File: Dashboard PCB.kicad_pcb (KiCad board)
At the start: 2 copper layers, 200 x 100 mm, 59 parts, among them J1 Controls_Leader_Export_02x06, J3 INDICATOR_SWITCH_OUT, J4 FAN_CTRL_01x02, J5 Horn_In_01x02, J6 Horn_Out_01x02

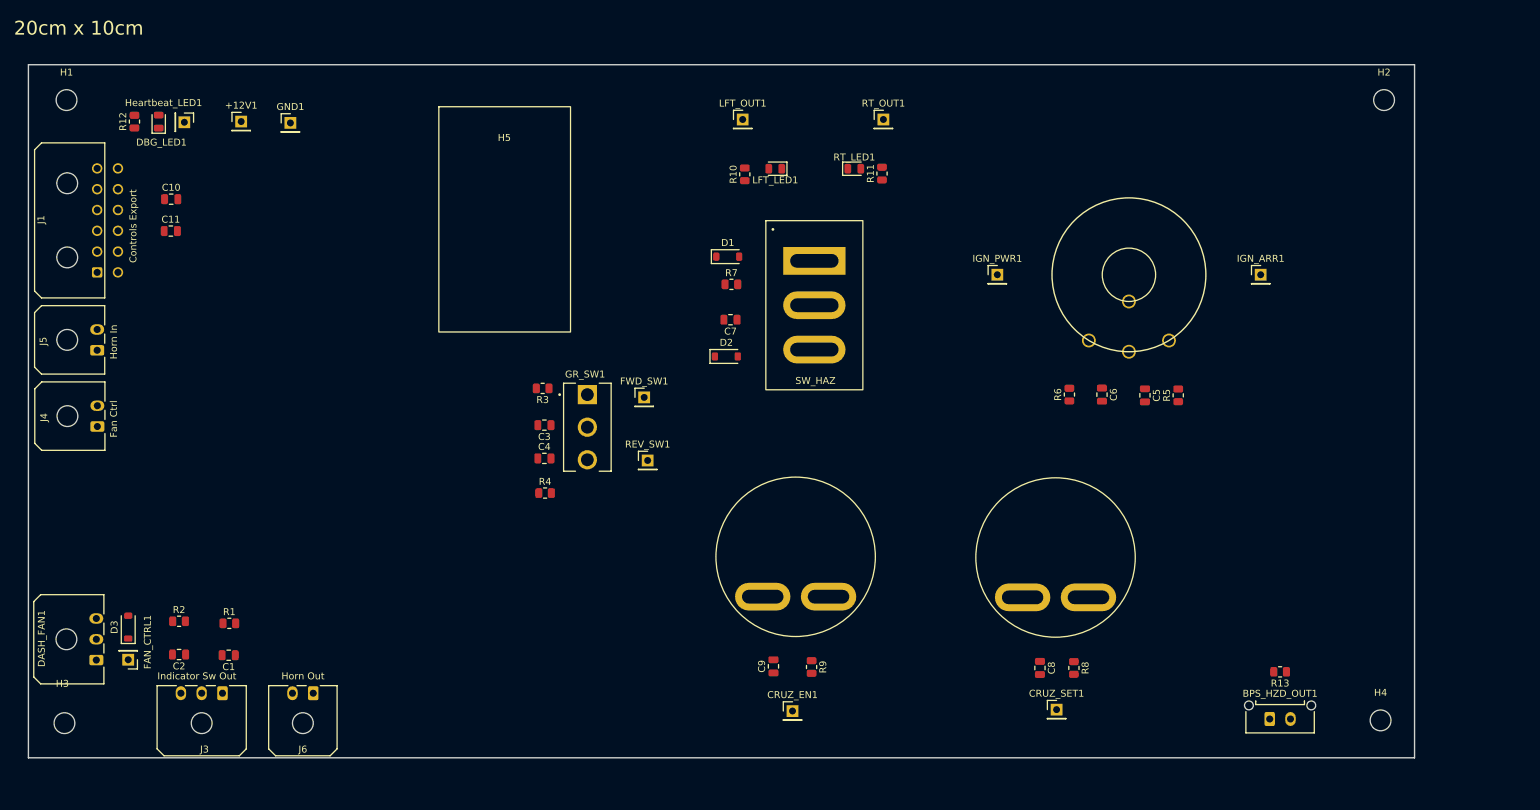
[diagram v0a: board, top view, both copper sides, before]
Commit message: Changed layout, added 3d models
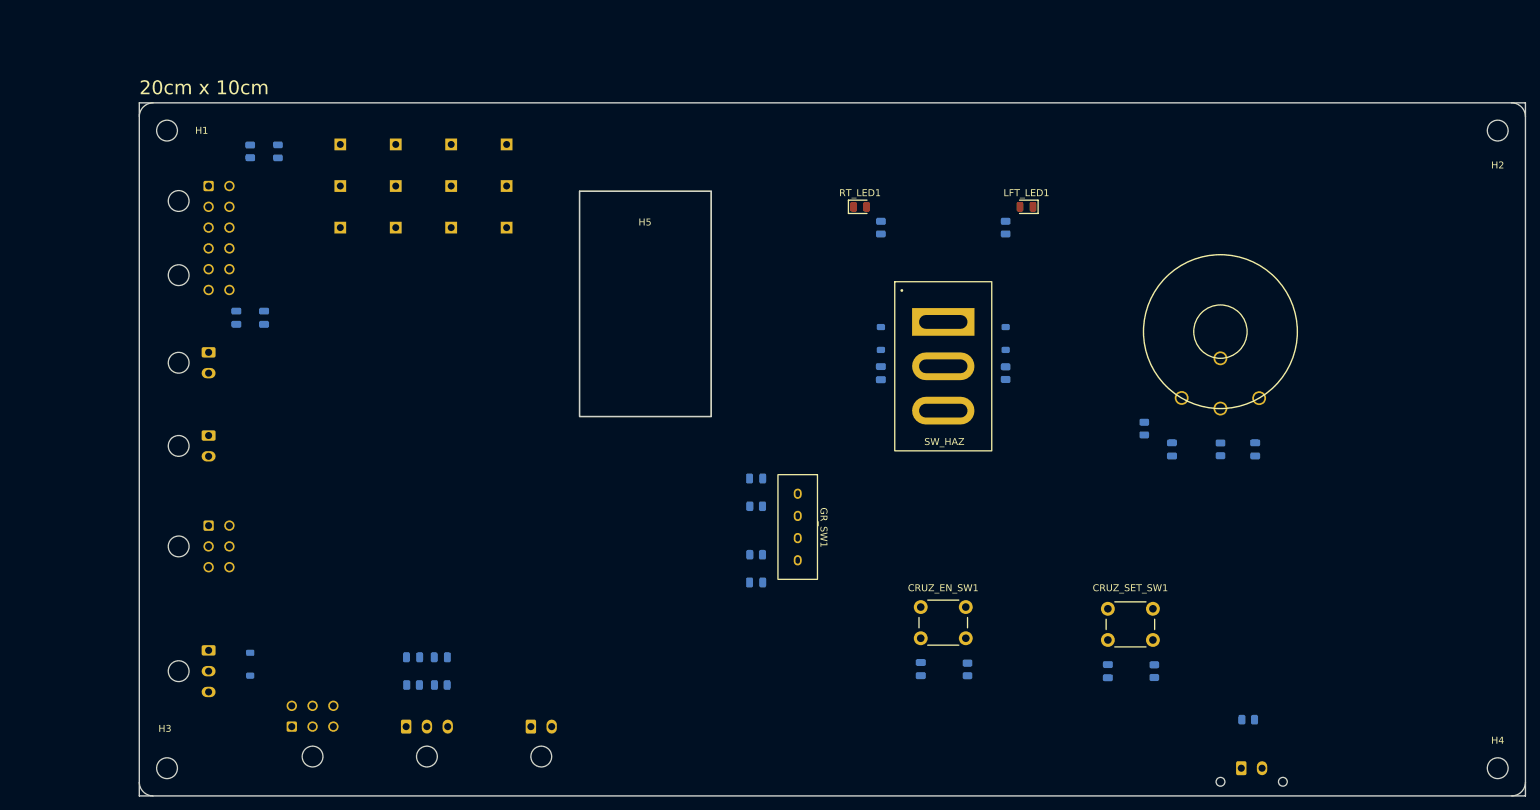
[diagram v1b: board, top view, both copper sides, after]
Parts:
- added J2: CAN, Connector_Molex:Molex_Micro-Fit_3.0_43045-0600_2x03_P3.00mm_Horizontal, B.Cu at (74.0, 104.0)
- added J7: CAN, Connector_Molex:Molex_Micro-Fit_3.0_43045-0600_2x03_P3.00mm_Horizontal, B.Cu at (86.0, 133.0)
- +12V1, BPS_HZD_OUT1, C1, C10, C11, C2, C3, C4, C5, C6, C7, C8, C9, CRUZ_EN1, CRUZ_SET1, D1, D2, D3, DASH_FAN1, DBG_LED1, FAN_CTRL1, FWD_SW1, GND1, Heartbeat_LED1, IGN_ARR1, IGN_PWR1, J1, J3, J4, J5, J6, LFT_OUT1, R1, R10, R11, R12, R13, R2, R3, R4, R5, R6, R7, R8, R9, REV_SW1, RT_OUT1: moved to B.Cu
- CRUZ_EN_SW1, CRUZ_SET_SW1: footprint switched:SW_Butt_) -> Button_Switch_THT:SW_PUSH_6mm
- GR_SW1: footprint switched:SW_100_SP3T-Vertical -> switched:3posSlideToggle
- moved IGN_ARR1 133.0 mm to (93.0, 61.0), turned to 180 degrees
- moved CRUZ_SET1 113.8 mm to (117.0, 49.0), turned to 180 degrees
- moved IGN_PWR1 95.7 mm to (93.0, 55.0), turned to 180 degrees
- moved CRUZ_EN1 86.3 mm to (117.0, 55.0), turned to 180 degrees
- moved FAN_CTRL1 73.3 mm to (101.0, 61.0), turned to -90 degrees
- moved RT_OUT1 56.6 mm to (117.0, 61.0), turned to 180 degrees
- moved LFT_OUT1 50.2 mm to (101.0, 49.0), turned to 180 degrees
- moved REV_SW1 48.7 mm to (109.0, 55.0), turned to 180 degrees
- moved R7 41.6 mm to (189.0, 82.0), turned to 90 degrees
- moved D2 40.4 mm to (189.0, 77.0), turned to -90 degrees
- moved R2 38.9 mm to (107.5, 127.0)
- moved R10 38.4 mm to (189.0, 61.0)
- moved C2 37.8 mm to (107.5, 123.0)
- moved FWD_SW1 37.1 mm to (109.0, 61.0), turned to 180 degrees
- moved LFT_LED1 36.7 mm to (192.0, 58.0)
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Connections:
- BPS_HZD_OUT1 pad 2: GND -> /BPS_HZD
- GR_SW1 pad 1: /FWD_SW -> +12V
- GR_SW1 pad 2: +12V -> /FWD_SW
- GR_SW1 pad 3: /REV_SW -> (no net)
- Heartbeat_LED1 pad 1: GND -> /DBG_LED
- R12 pad 1: /DBG_LED -> +12V
- R13 pad 1: /BPS_HZD -> +12V
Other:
- outline, holes or cut-outs redrawn
- board text added: "Approx 3d model"
- board text added: "Placeholder 3d model"
